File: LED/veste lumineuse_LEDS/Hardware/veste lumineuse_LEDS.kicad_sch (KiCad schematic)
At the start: 2 parts, among them U1 STM32G431KBTx, U2 CH224K

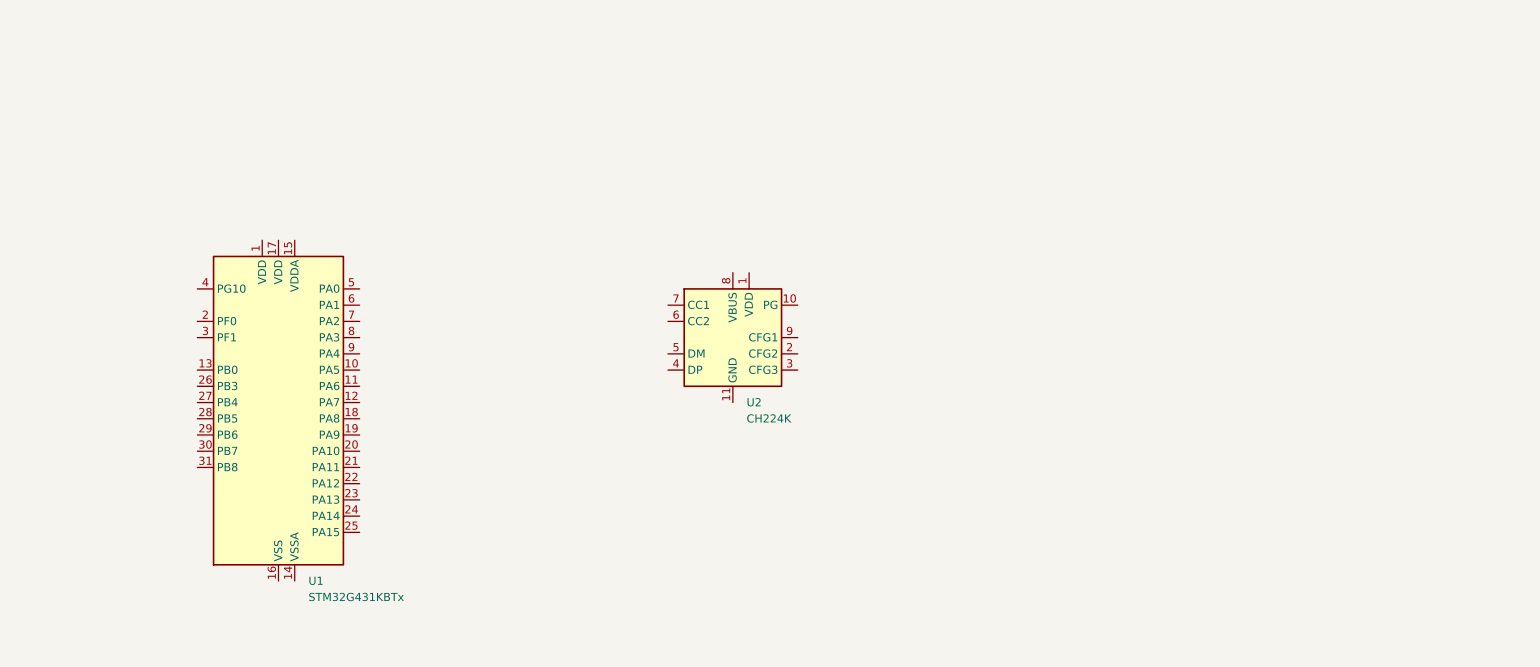
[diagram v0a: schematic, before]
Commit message: schema kicad 10_03_25 1
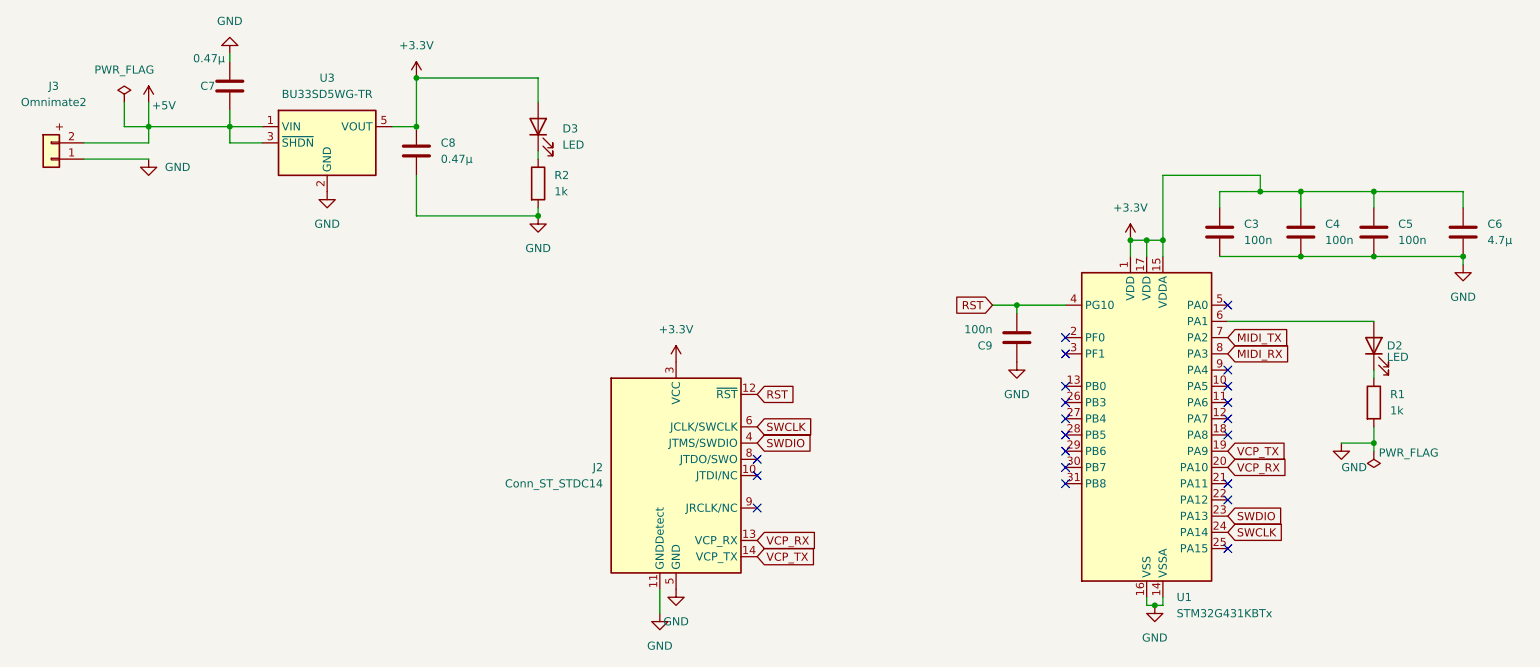
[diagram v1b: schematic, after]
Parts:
- removed U2: CH224K, Package_SO:SSOP-10-1EP_3.9x4.9mm_P1mm_EP2.1x3.3mm, symbol Interface_USB:CH224K
- added C3, C4, C5, C9: 100n, FootprintGamelGe2_v8.0:C_Rect_L7.0mm_W2.5mm_P5.00mm, symbol SymbGamelGe2_v8.0:C
- added C6: 4.7µ, FootprintGamelGe2_v8.0:C_Rect_L7.0mm_W2.5mm_P5.00mm, symbol SymbGamelGe2_v8.0:C
- added C7, C8: 0.47µ, FootprintGamelGe2_v8.0:C_Rect_L7.0mm_W2.5mm_P5.00mm, symbol SymbGamelGe2_v8.0:C
- added D2, D3: LED, LED_SMD:LED_0201_0603Metric, symbol Device:LED
- added J2: Conn_ST_STDC14, symbol Connector:Conn_ST_STDC14
- added J3: Omnimate2, FootprintGamelGe2_v8.0:OmnimateSL-5,08_1x02_P5.08mm_Vertical, symbol SymbGamelGe2_v8.0:Omnimate2
- added R1, R2: 1k, FootprintGamelGe2_v8.0:R_Axial_DIN0207_L6.3mm_D2.5mm_P10.16mm_Horizontal, symbol SymbGamelGe2_v8.0:R
- added U3: BU33SD5WG-TR, Package_TO_SOT_SMD:SOT-23-5, symbol Regulator_Linear:MCP1802x-xx02xOT
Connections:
- net +3.3V: now reaches U1.1 (VDD)
- net +3.3V: now also U1.15 (VDDA), U1.17 (VDD), C3.1, C4.1, C5.1, C6.1, C8.1, D3.2 (A), J2.3 (VCC), U3.5 (VOUT)
- net GND: now reaches U1.14 (VSSA)
- net GND: now also U1.16 (VSS), U1.32 (VSS), C3.2, C4.2, C5.2, C6.2, C7.2, C8.2, C9.1, J2.11 (GNDDetect), J2.5 (GND), J2.7 (GND), J3.1 (Pin_1), R1.2, R2.2, U3.2 (GND)
- net VCP_TX: now reaches U1.19 (PA9)
- net VCP_TX: now also J2.14 (VCP_TX)
- net VCP_RX: now reaches U1.20 (PA10)
- net VCP_RX: now also J2.13 (VCP_RX)
- net SWDIO: now reaches U1.23 (PA13)
- net SWDIO: now also J2.4 (JTMS/SWDIO)
- net SWCLK: now reaches U1.24 (PA14)
- net SWCLK: now also J2.6 (JCLK/SWCLK)
- net RST: now reaches U1.4 (PG10)
- net RST: now also C9.2, J2.12 (~{RST})
- net at U1.6 (PA1): now also D2.2 (A)
- net MIDI_TX: now reaches U1.7 (PA2)
- net MIDI_RX: now reaches U1.8 (PA3)
- new net: D2.1 (K), R1.1
- new net: D3.1 (K), R2.1
- new net +5V: C7.1, J3.2 (Pin_2), U3.1 (VIN), U3.3 (~{SHDN})
- no-connect marks 0 -> 21
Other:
- moved on the sheet: U1
